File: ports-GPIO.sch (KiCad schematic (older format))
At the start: 44 parts, among them J1 Conn_01x20_Male, J2 HDMI_A, J3 Conn_01x20_Male, Q1 MMBT3906, Q2 MMBT3906, Q3 MMBT3906, Q4 MMBT3904, Q5 MMBT3906, Q6 MMBT3904

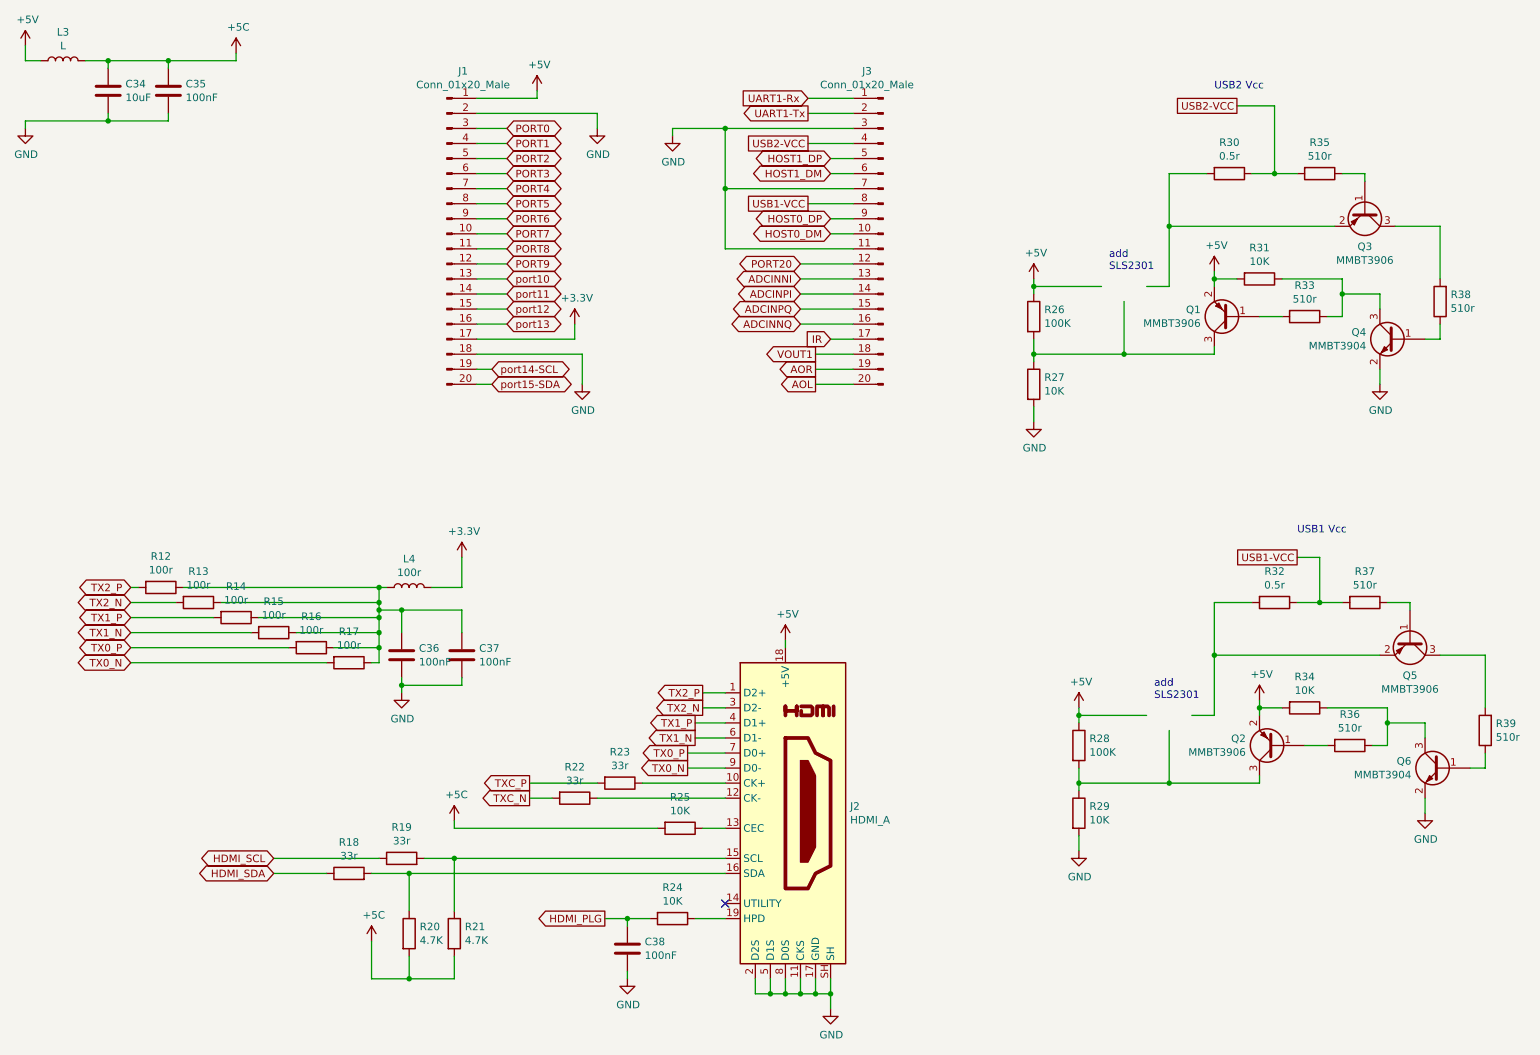
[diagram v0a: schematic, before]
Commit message: added todo list before i feel aleeped on my keybard*
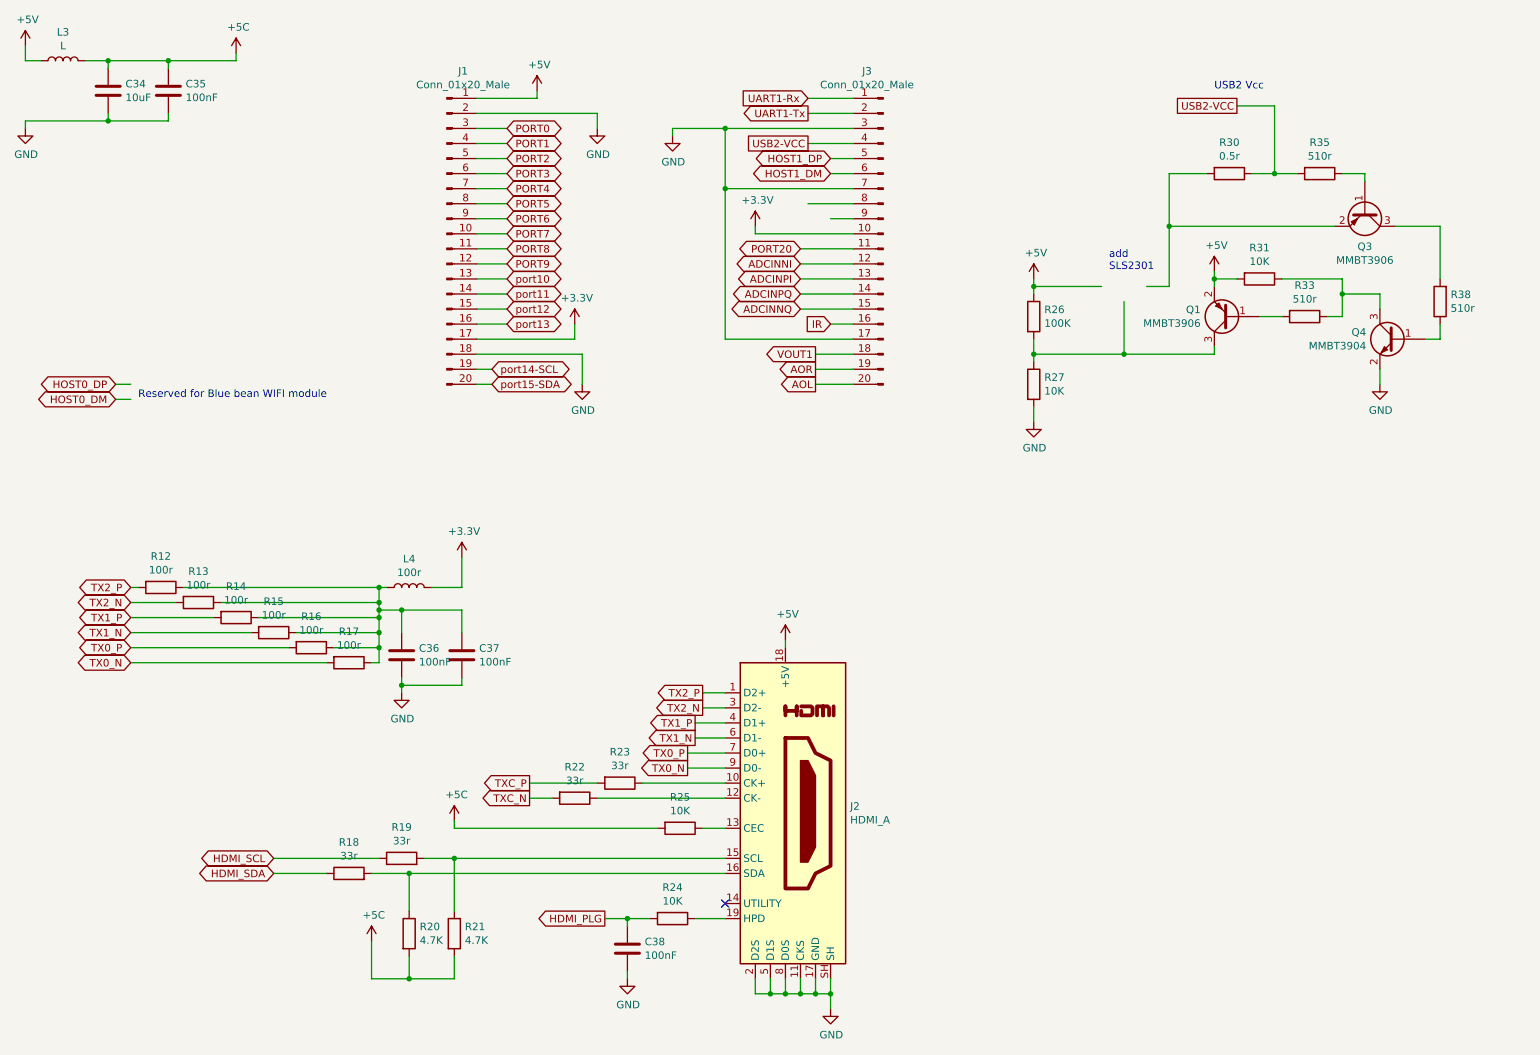
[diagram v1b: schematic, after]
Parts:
- removed Q2, Q5: MMBT3906, Package_TO_SOT_SMD:SOT-23, symbol Transistor_BJT:MMBT3906
- removed Q6: MMBT3904, Package_TO_SOT_SMD:SOT-23, symbol Transistor_BJT:MMBT3904
- removed R28: 100K, symbol Device:R
- removed R29, R34: 10K, symbol Device:R
- removed R32: 0.5r, symbol Device:R
- removed R36, R37, R39: 510r, symbol Device:R
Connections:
- net labels removed: USB1-VCC
- wire segments 206 -> 173
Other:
- note added: "Reserved for Blue bean WIFI module"
- note removed: "USB1 Vcc"

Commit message: finished scimatic for now, and started populating PCB. *chugs rrum*
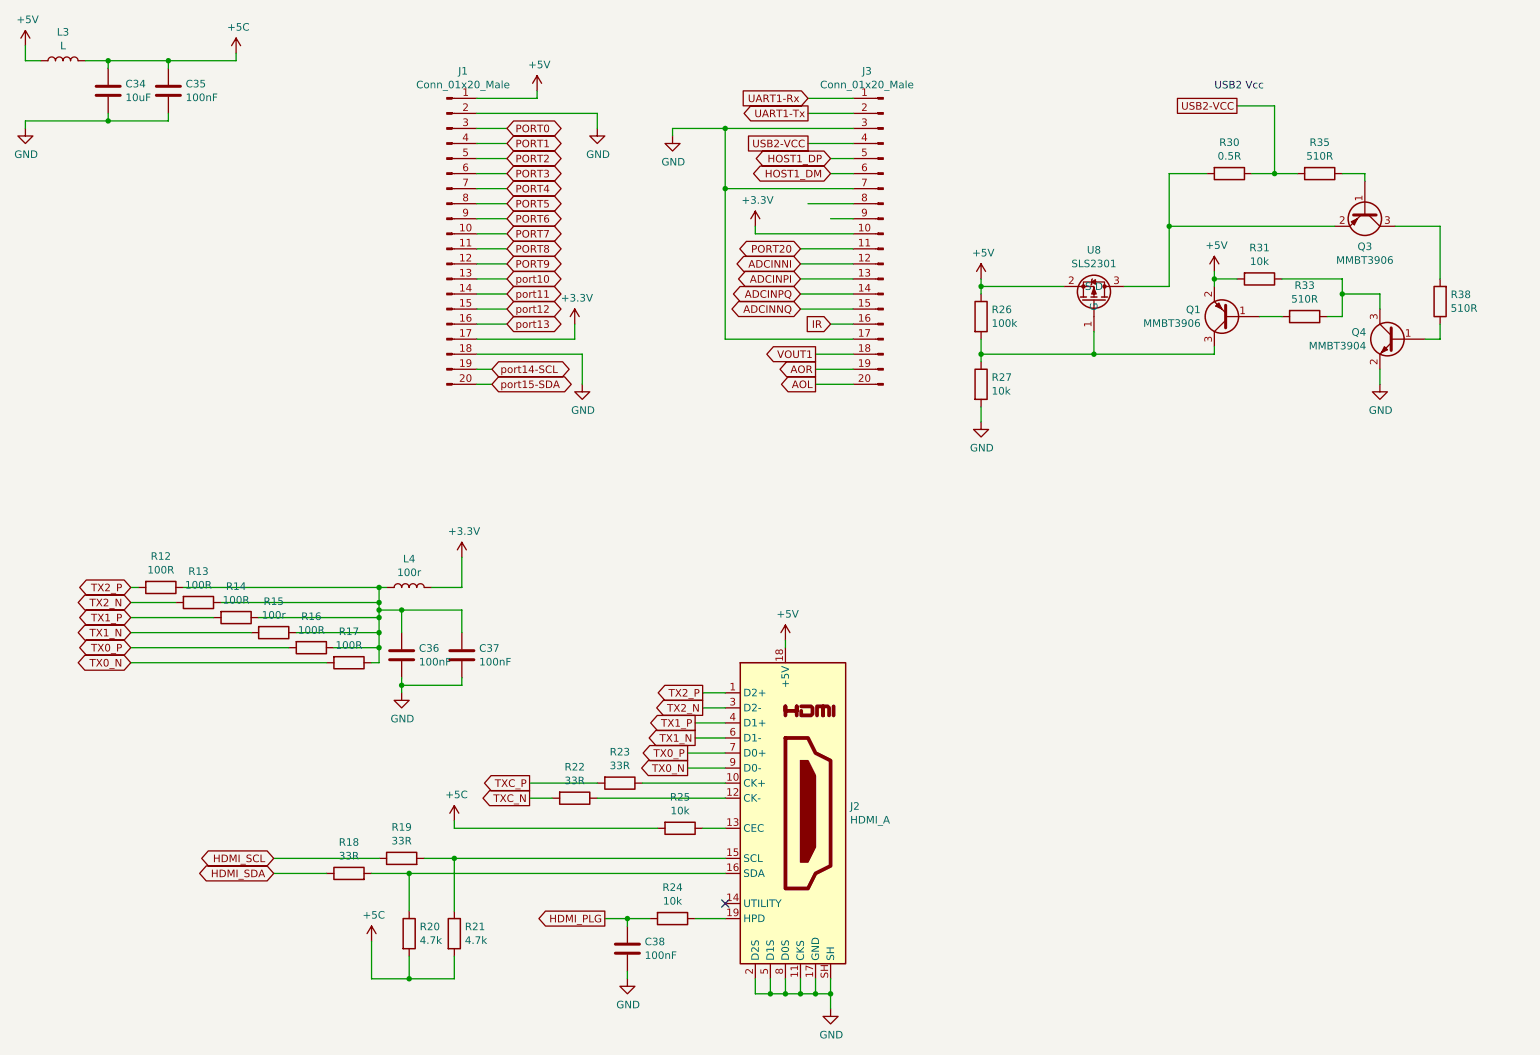
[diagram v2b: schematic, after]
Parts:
- added U8: SLS2301, Package_TO_SOT_SMD:SOT-23, symbol Csky:SLS2301
- C34, C35, C36, C37, C38: footprint (none) -> Capacitor_SMD:C_0402_1005Metric
- J1, J3: footprint (none) -> Connector_PinSocket_2.54mm:PinSocket_1x20_P2.54mm_Vertical
- J2: footprint (none) -> Connector_HDMI:HDMI_Micro-D_Molex_46765-0x01
- L3, L4: footprint (none) -> Inductor_SMD:L_0402_1005Metric
- R12, R13, R14, R16, R17: value 100r -> 100R; footprint (none) -> Resistor_SMD:R_0402_1005Metric
- R15: footprint (none) -> Resistor_SMD:R_0402_1005Metric
- R18, R19, R22, R23: value 33r -> 33R; footprint (none) -> Resistor_SMD:R_0402_1005Metric
- R20, R21: value 4.7K -> 4.7k; footprint (none) -> Resistor_SMD:R_0402_1005Metric
- R24, R25, R27, R31: value 10K -> 10k; footprint (none) -> Resistor_SMD:R_0402_1005Metric
- R26: value 100K -> 100k; footprint (none) -> Resistor_SMD:R_0402_1005Metric
- R30: value 0.5r -> 0.5R; footprint (none) -> Resistor_SMD:R_0402_1005Metric
- R33, R35, R38: value 510r -> 510R; footprint (none) -> Resistor_SMD:R_0402_1005Metric
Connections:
- net labels removed: HOST0_DM, HOST0_DP
- wire segments 173 -> 171
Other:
- note removed: "Reserved for Blue bean WIFI module"
- note removed: "add\nSLS2301"
- moved on the sheet: R26, R27
